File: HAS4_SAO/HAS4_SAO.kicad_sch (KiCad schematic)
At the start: 7 parts, among them SW1 MLL1200S, X1 Badgelife_sao_connector_v169b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

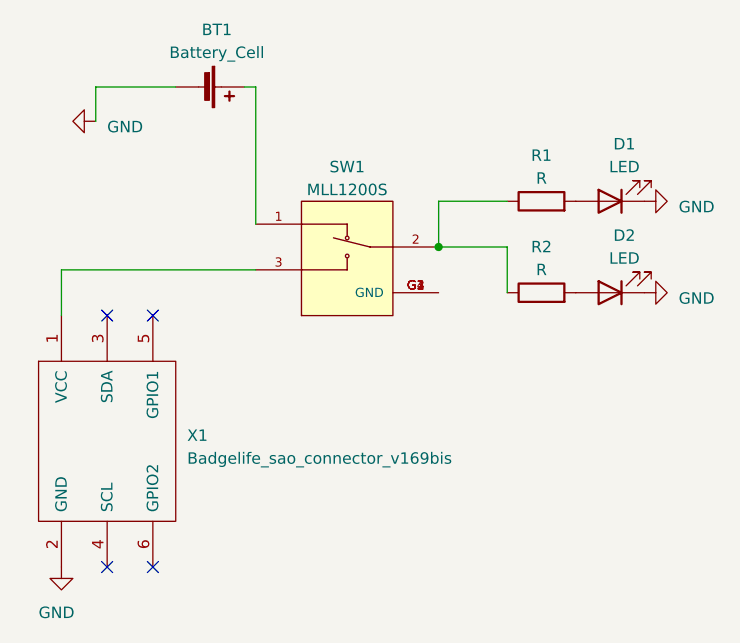
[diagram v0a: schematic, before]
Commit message: HAS4 SAO for DC31
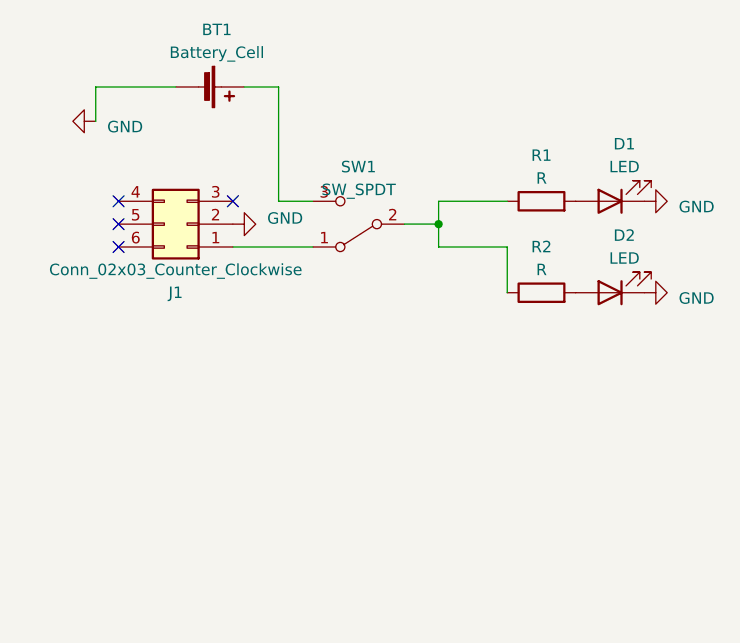
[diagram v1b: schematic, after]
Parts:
- removed SW1: MLL1200S, SW_MLL1200S, symbol MLL1200S:MLL1200S
- removed X1: Badgelife_sao_connector_v169bis, Connector_PinHeader_2.54mm:PinHeader_2x03_P2.54mm_Vertical, symbol badgelife_shitty_addon_v169bis:Badgelife_sao_connector_v169bis
- added J1: Conn_02x03_Counter_Clockwise, Connector_PinHeader_2.54mm:PinHeader_2x03_P2.54mm_Vertical, symbol Connector_Generic:Conn_02x03_Counter_Clockwise
- added SW1: SW_SPDT, Button_Switch_SMD:SW_SPDT_PCM12, symbol Switch:SW_SPDT
- BT1: footprint Battery:BatteryHolder_Keystone_1058_1x2032 -> Battery:BatteryHolder_Keystone_3034_1x20mm
- D1, D2: footprint LED_SMD:LED_0805_2012Metric_Pad1.15x1.40mm_HandSolder -> LED_SMD:LED_0805_2012Metric
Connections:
- net GND: now also J1.2 (Pin_2)
- net at R1.1, R2.1: now also SW1.2 (B)
- net at BT1.1 (+): now also SW1.3 (C)
- new net: J1.1 (Pin_1), SW1.1 (A)
